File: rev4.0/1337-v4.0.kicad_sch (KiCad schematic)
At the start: 63 parts, among them J1 USB_IN, J2 AVR-ISP-6, SW1 SW_Push, SW2 EC11, U2 USBLC6-2SC6, U3 ATMEGA32U4, U5 SSD1306, Y2 16MHz

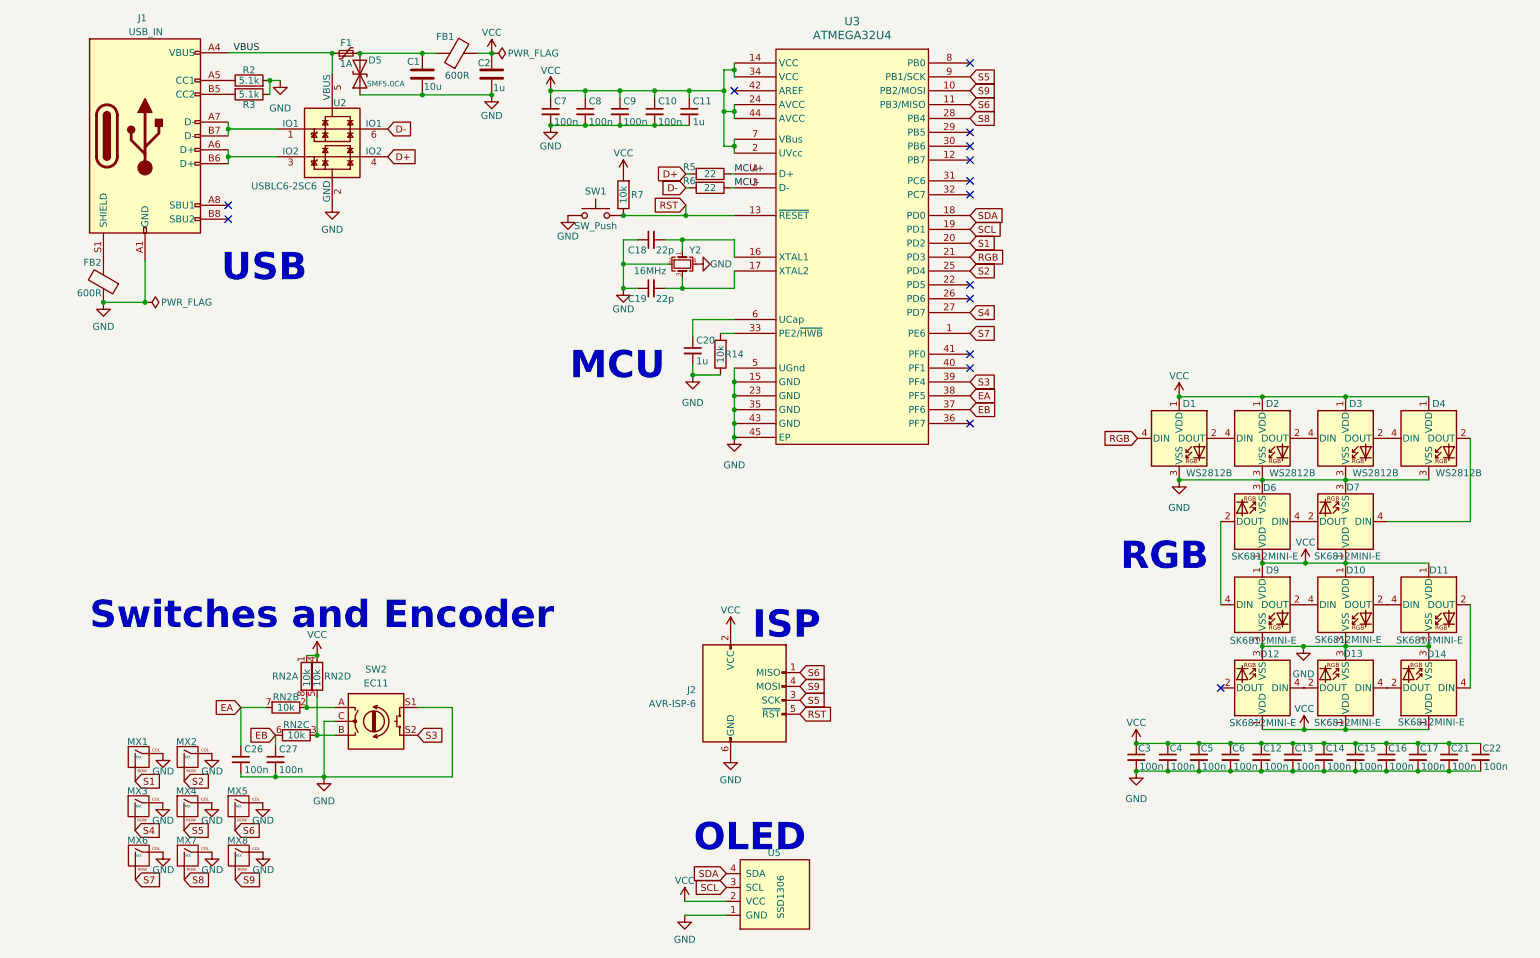
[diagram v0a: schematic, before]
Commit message: traced PCB
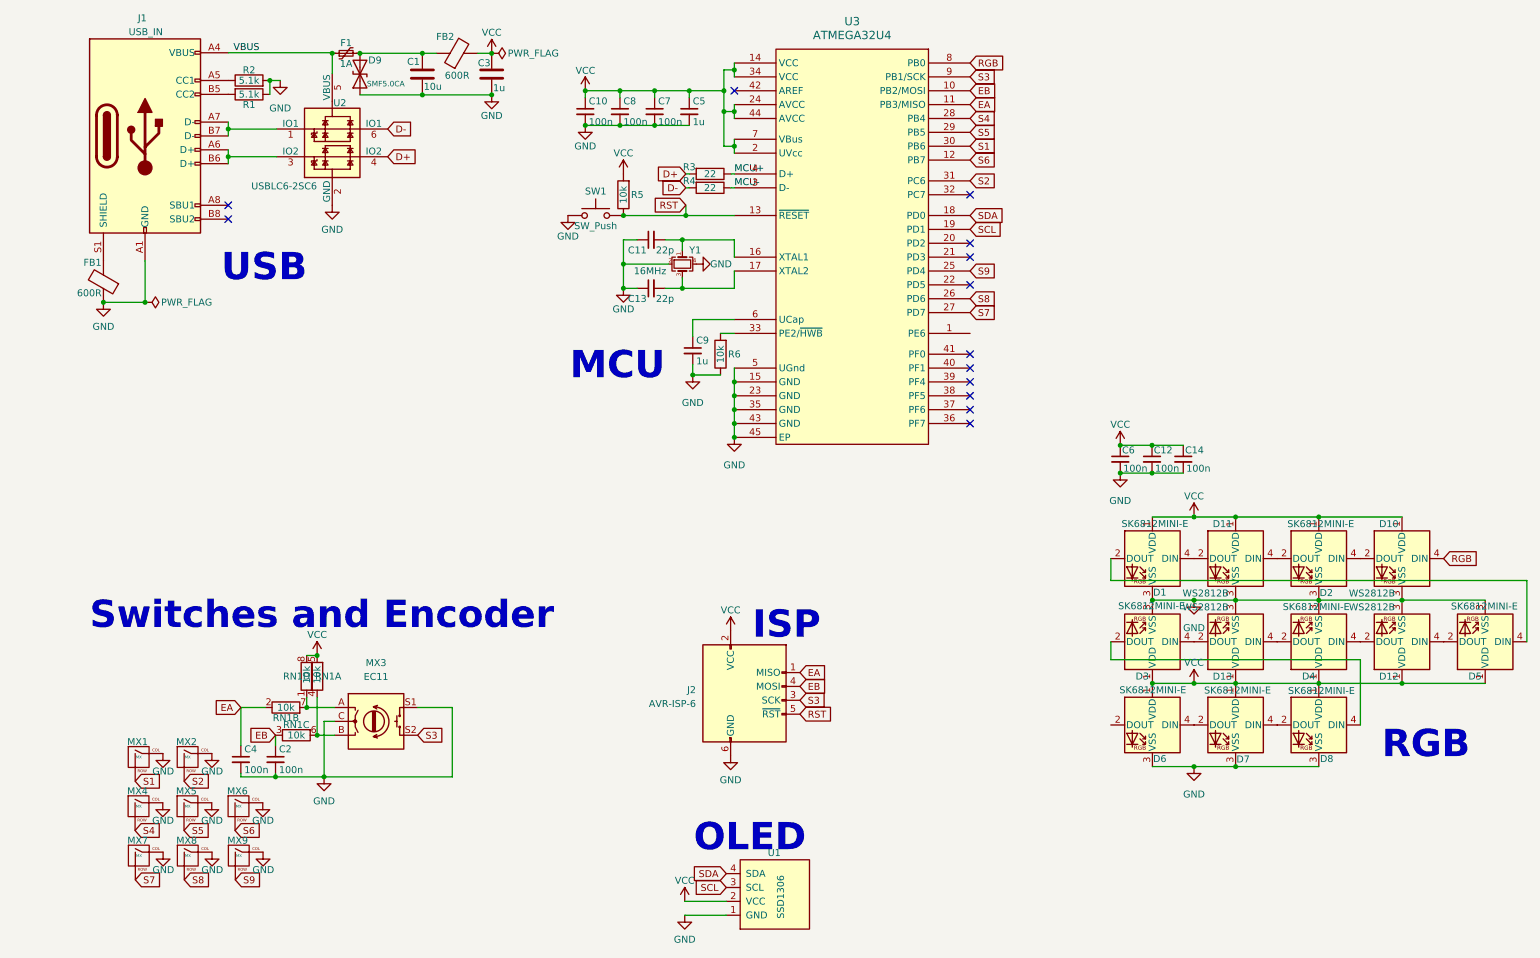
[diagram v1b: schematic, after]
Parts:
- removed C12, C14, C15, C16, C17, C21, C22, C4, C6, C7: 100n, Capacitor_SMD:C_0603_1608Metric, symbol Device:C_Small
- MX3: renamed from SW2; footprint Rotary_Encoder:RotaryEncoder_Alps_EC11E-Switch_Vertical_H20mm -> 0xcb:EC11
- renumbered C8 to C10, C18 to C11, C5 to C12, C19 to C13, C13 to C14, C27 to C2, C2 to C3, C26 to C4, C11 to C5, C3 to C6, C10 to C7, C9 to C8, C20 to C9, D6 to D1, D2 to D10, D1 to D11, D4 to D12, D3 to D13, D7 to D2, D9 to D3, D10 to D4, D11 to D5, D12 to D6, D13 to D7, D14 to D8, D5 to D9, FB2 to FB1, FB1 to FB2, MX3 to MX4, MX4 to MX5, MX5 to MX6, MX6 to MX7, MX7 to MX8, MX8 to MX9, R3 to R1, R5 to R3, R6 to R4, R7 to R5, R14 to R6, RN2 to RN1, U5 to U1, Y2 to Y1
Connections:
- net EA: now also J2.1 (MISO), RN1.2 (R2.1), U3.11 (PB3/MISO); no longer RN1.7 (R2.2), U3.38 (PF5)
- net EB: now also J2.4 (MOSI), RN1.3 (R3.1), U3.10 (PB2/MOSI); no longer RN1.6 (R3.2), U3.37 (PF6)
- net RGB: now also D10.4 (DIN), U3.8 (PB0); no longer D11.4 (DIN), U3.21 (PD3)
- net S1: now also U3.30 (PB6); no longer U3.20 (PD2)
- net S2: now also U3.31 (PC6); no longer U3.25 (PD4)
- net S3: now also J2.3 (SCK), U3.9 (PB1/SCK); no longer U3.39 (PF4)
- net S4: now also U3.28 (PB4); no longer U3.27 (PD7)
- net S5: now also U3.29 (PB5); no longer J2.3 (SCK), U3.9 (PB1/SCK)
- net S6: now also U3.12 (PB7); no longer J2.1 (MISO), U3.11 (PB3/MISO)
- net S7: now also U3.27 (PD7); no longer U3.1 (PE6)
- net S8: now also U3.26 (PD6); no longer U3.28 (PB4)
- net S9: now also U3.25 (PD4); no longer J2.4 (MOSI), U3.10 (PB2/MOSI)
- net VCC: now also RN1.5 (R4.2), RN1.8 (R1.2); no longer RN1.1 (R1.1), RN1.4 (R4.1)
- net at D1.2 (DOUT): now also D5.4 (DIN); no longer D3.4 (DIN)
- net at D1.4 (DIN): now also D11.2 (DOUT); no longer D2.2 (DOUT)
- net at D10.2 (DOUT): now also D2.4 (DIN); no longer D13.4 (DIN)
- net at D13.2 (DOUT): now also D3.4 (DIN); no longer D12.4 (DIN)
- net at D3.2 (DOUT): now also D8.4 (DIN); no longer D4.4 (DIN)
- net at D5.2 (DOUT): now also D12.4 (DIN); no longer D8.4 (DIN)
- net at D4.2 (DOUT): now also D13.4 (DIN); no longer D5.4 (DIN)
- net at D12.2 (DOUT): now also D4.4 (DIN); no longer D2.4 (DIN)
- new net: MX3.B, RN1.4 (R4.1), RN1.6 (R3.2)
- new net: MX3.A, RN1.1 (R1.1), RN1.7 (R2.2)
- new net: D11.4 (DIN), D2.2 (DOUT)
- no-connect marks 15 -> 13
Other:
- moved on the sheet: C12, C14, C6, D1, D10, D11, D12, D13, D2, D3, D4, D5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

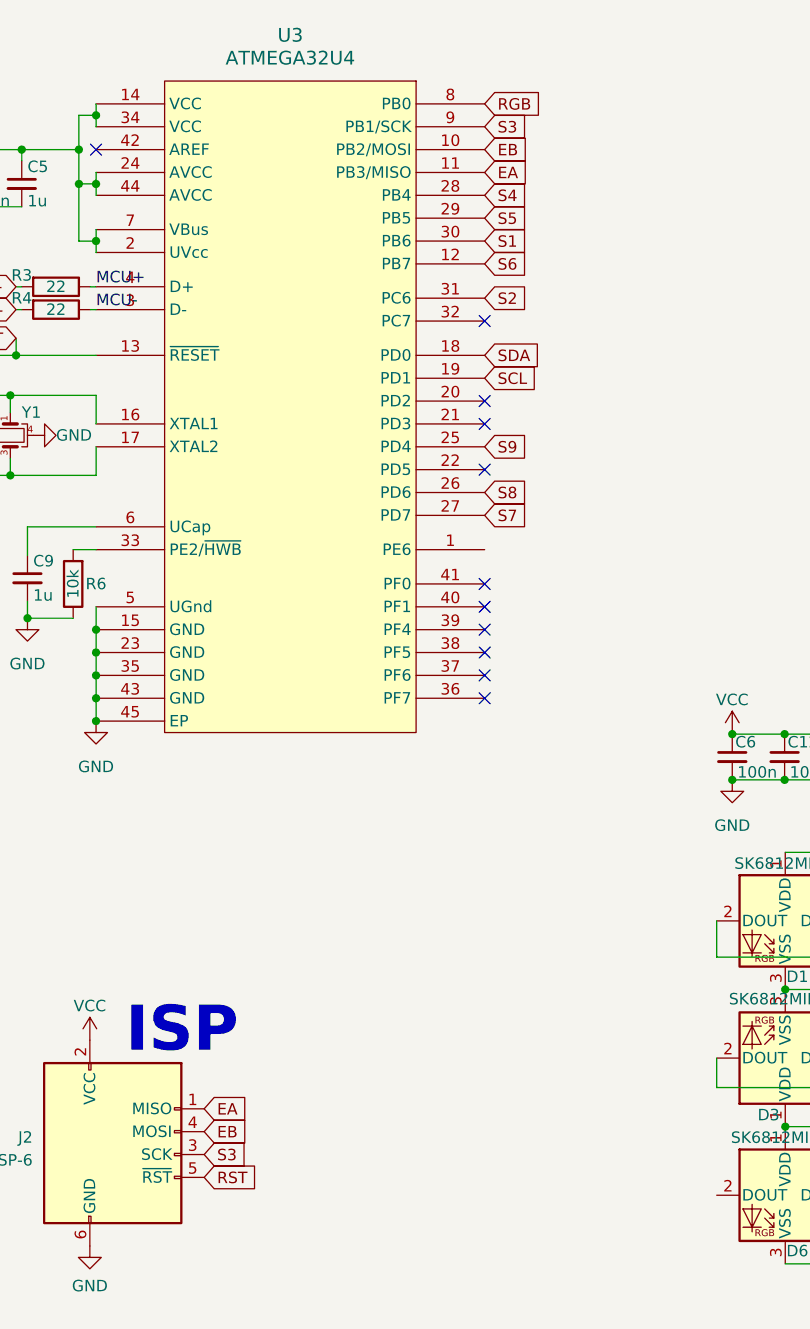
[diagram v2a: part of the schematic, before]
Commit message: finalizing v4.0
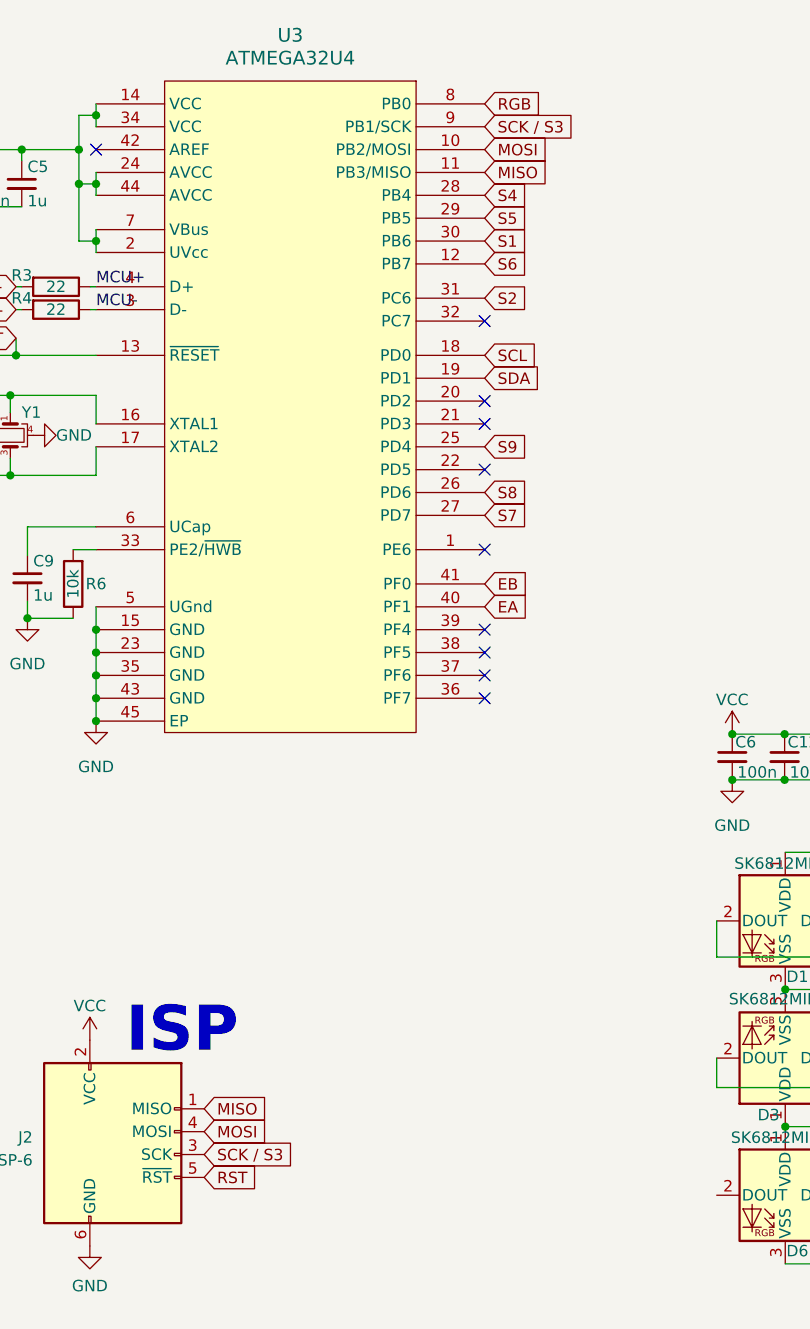
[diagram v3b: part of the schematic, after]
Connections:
- net EA: now also U3.40 (PF1); no longer J2.1 (MISO), U3.11 (PB3/MISO)
- net EB: now also U3.41 (PF0); no longer J2.4 (MOSI), U3.10 (PB2/MOSI)
- net S3: no longer J2.3 (SCK), U3.9 (PB1/SCK)
- net SCL: now also U3.18 (PD0); no longer U3.19 (PD1)
- net SDA: now also U3.19 (PD1); no longer U3.18 (PD0)
- new net MISO: J2.1 (MISO), U3.11 (PB3/MISO)
- new net MOSI: J2.4 (MOSI), U3.10 (PB2/MOSI)
- new net SCK / S3: J2.3 (SCK), U3.9 (PB1/SCK)
- no-connect marks 13 -> 12
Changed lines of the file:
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@@
   (no_connect (at 176.53 51.4096))
   (no_connect (at 176.53 67.9196))
-  (no_connect (at 176.53 80.6196))
-  (no_connect (at 176.53 83.1596))
   (no_connect (at 176.53 93.3196))
   (no_connect (at 40.64 53.34))
@@
   (no_connect (at 176.53 90.7796))
   (no_connect (at 176.53 62.8396))
+  (no_connect (at 176.53 76.8096))
   (wire (pts (xy 240.411 140.9192) (xy 255.651 140.9192))
     (stroke (width 0) (type default) (color 0 0 0 0))
@@
     )
   )
-  (global_label "SDA" (shape input) (at 176.53 55.2196 0) (fields_autoplaced)
-    (effects (font (size 1.27 1.27)) (justify left))
-    (property "Intersheet References" "${INTERSHEET_REFS}" (id 0) (at 182.5112 55.1402 0)
+  (global_label "SDA" (shape input) (at 176.53 57.7596 0) (fields_autoplaced)
+    (effects (font (size 1.27 1.27)) (justify left))
+    (property "Intersheet References" "${INTERSHEET_REFS}" (id 0) (at 182.5112 57.6802 0)
       (effects (font (size 1.27 1.27)) (justify left) hide)
     )
@@
     )
   )
-  (global_label "EA" (shape input) (at 176.53 34.8996 0) (fields_autoplaced)
-    (effects (font (size 1.27 1.27)) (justify left))
-    (property "Intersheet References" "${INTERSHEET_REFS}" (id 0) (at 181.1807 34.8202 0)
+  (global_label "MISO" (shape input) (at 176.53 34.8996 0) (fields_autoplaced)
+    (effects (font (size 1.27 1.27)) (justify left))
+    (property "Intersheet References" "${INTERSHEET_REFS}" (id 0) (at 183.7298 34.8202 0)
       (effects (font (size 1.27 1.27)) (justify left) hide)
     )
@@
     )
   )
-  (global_label "SCL" (shape input) (at 176.53 57.7596 0) (fields_autoplaced)
-    (effects (font (size 1.27 1.27)) (justify left))
-    (property "Intersheet References" "${INTERSHEET_REFS}" (id 0) (at 182.4507 57.6802 0)
+  (global_label "SCL" (shape input) (at 176.53 55.2196 0) (fields_autoplaced)
+    (effects (font (size 1.27 1.27)) (justify left))
+    (property "Intersheet References" "${INTERSHEET_REFS}" (id 0) (at 182.4507 55.1402 0)
+      (effects (font (size 1.27 1.27)) (justify left) hide)
+    )
+  )
+  (global_label "EA" (shape input) (at 176.53 83.1596 0) (fields_autoplaced)
+    (effects (font (size 1.27 1.27)) (justify left))
+    (property "Intersheet References" "${INTERSHEET_REFS}" (id 0) (at 181.1807 83.0802 0)
       (effects (font (size 1.27 1.27)) (justify left) hide)
     )
@@
     )
   )
-  (global_label "EA" (shape input) (at 145.3642 138.938 0) (fields_autoplaced)
-    (effects (font (size 1.27 1.27)) (justify left))
-    (property "Intersheet References" "${INTERSHEET_REFS}" (id 0) (at 150.0149 138.8586 0)
+  (global_label "EB" (shape input) (at 176.53 80.6196 0) (fields_autoplaced)
+    (effects (font (size 1.27 1.27)) (justify left))
+    (property "Intersheet References" "${INTERSHEET_REFS}" (id 0) (at 181.3621 80.5402 0)
+      (effects (font (size 1.27 1.27)) (justify left) hide)
+    )
+  )
+  (global_label "MISO" (shape input) (at 145.3642 138.938 0) (fields_autoplaced)
+    (effects (font (size 1.27 1.27)) (justify left))
+    (property "Intersheet References" "${INTERSHEET_REFS}" (id 0) (at 152.564 138.8586 0)
       (effects (font (size 1.27 1.27)) (justify left) hide)
     )
@@
     )
   )
-  (global_label "S3" (shape input) (at 176.53 29.8196 0) (fields_autoplaced)
-    (effects (font (size 1.27 1.27)) (justify left))
-    (property "Intersheet References" "${INTERSHEET_REFS}" (id 0) (at 181.3621 29.7402 0)
+  (global_label "SCK {slash} S3" (shape input) (at 176.53 29.8196 0) (fields_autoplaced)
+    (effects (font (size 1.27 1.27)) (justify left))
+    (property "Intersheet References" "${INTERSHEET_REFS}" (id 0) (at 188.5679 29.7402 0)
       (effects (font (size 1.27 1.27)) (justify left) hide)
     )
@@
     )
   )
-  (global_label "S3" (shape input) (at 145.3642 144.018 0) (fields_autoplaced)
-    (effects (font (size 1.27 1.27)) (justify left))
-    (property "Intersheet References" "${INTERSHEET_REFS}" (id 0) (at 150.1963 143.9386 0)
+  (global_label "SCK {slash} S3" (shape input) (at 145.3642 144.018 0) (fields_autoplaced)
+    (effects (font (size 1.27 1.27)) (justify left))
+    (property "Intersheet References" "${INTERSHEET_REFS}" (id 0) (at 157.4021 143.9386 0)
       (effects (font (size 1.27 1.27)) (justify left) hide)
     )
@@
     )
   )
-  (global_label "EB" (shape input) (at 145.3642 141.478 0) (fields_autoplaced)
-    (effects (font (size 1.27 1.27)) (justify left))
-    (property "Intersheet References" "${INTERSHEET_REFS}" (id 0) (at 150.1963 141.3986 0)
-      (effects (font (size 1.27 1.27)) (justify left) hide)
-    )
-  )
-  (global_label "EB" (shape input) (at 176.53 32.3596 0) (fields_autoplaced)
-    (effects (font (size 1.27 1.27)) (justify left))
-    (property "Intersheet References" "${INTERSHEET_REFS}" (id 0) (at 181.3621 32.2802 0)
-      (effects (font (size 1.27 1.27)) (justify left) hide)
-    )
+  (global_label "MOSI" (shape input) (at 145.3642 141.478 0) (fields_autoplaced)
+    (effects (font (size 1.27 1.27)) (justify left))
+    (property "Intersheet References" "${INTERSHEET_REFS}" (id 0) (at 152.564 141.3986 0)
+      (effects (font (size 1.27 1.27)) (justify left) hide)
+    )
+  )
+  (global_label "MOSI" (shape input) (at 176.53 32.3596 0) (fields_autoplaced)
+    (effects (font (size 1.27 1.27)) (justify left))
+    (property "Intersheet References" "${INTERSHEET_REFS}" (id 0) (at 183.7298 32.2802 0)
+      (effects (font (size 1.27 1.27)) (justify left) hide)
+    )
